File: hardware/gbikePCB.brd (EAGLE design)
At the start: 26.7 x 28.3 mm, 19 parts, among them Q1 16M, U1 nRF51822

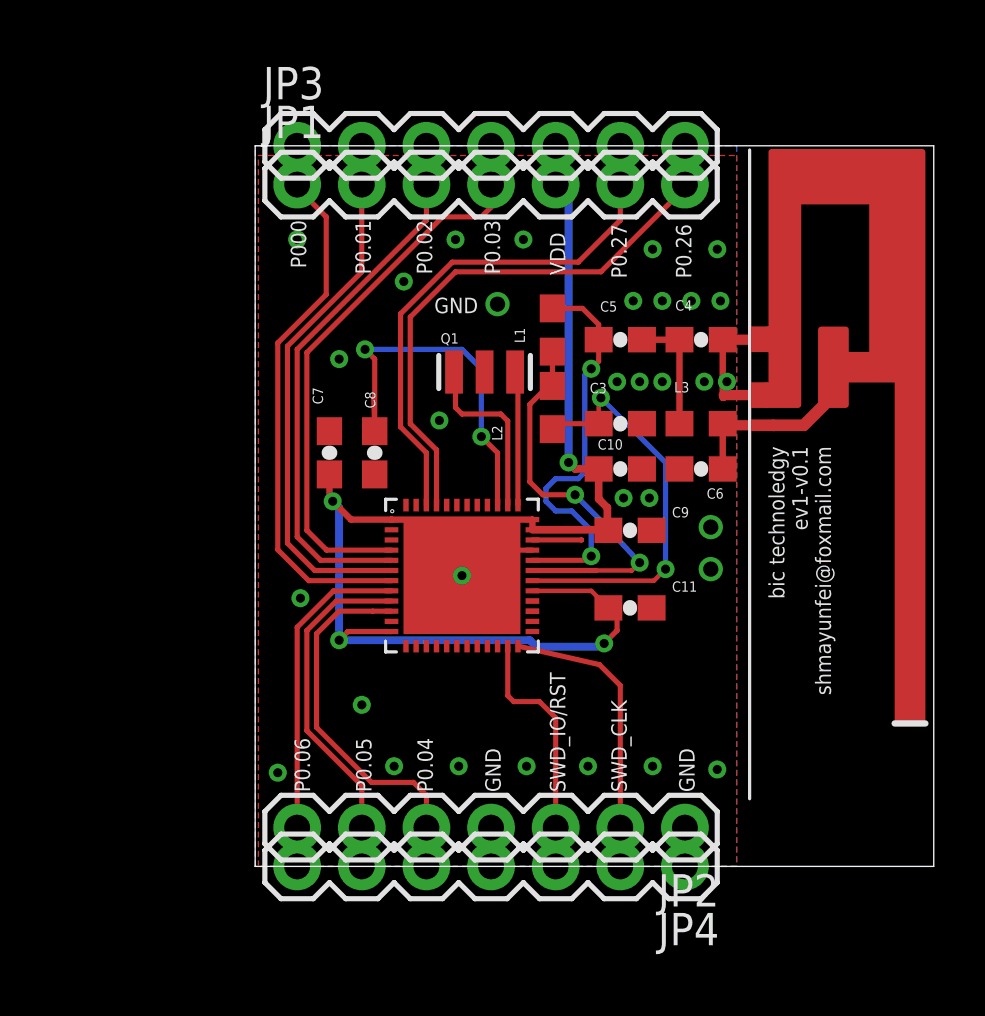
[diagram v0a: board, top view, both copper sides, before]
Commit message: updated pcb file
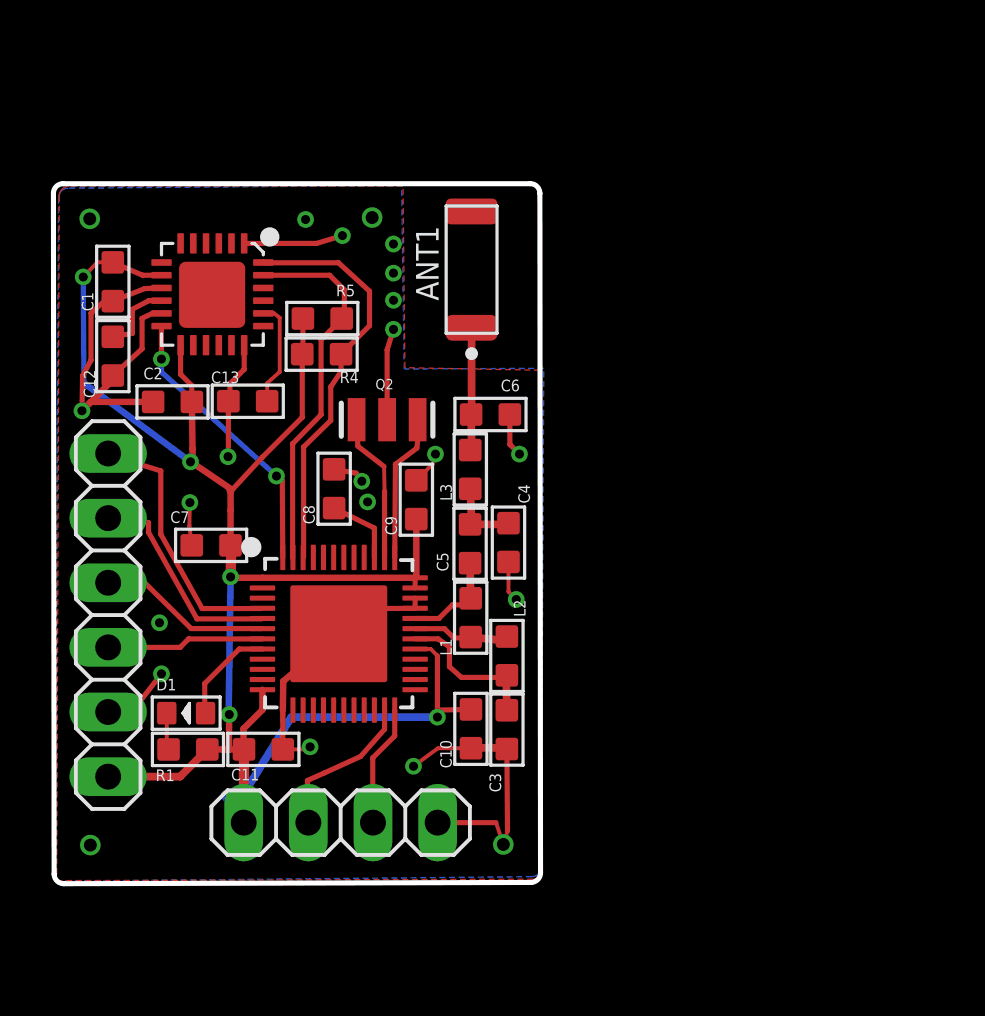
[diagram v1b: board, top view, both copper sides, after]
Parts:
- removed JP3, JP4: (no value), AUSER KJ:1X07
- removed Q1: 16M, APM_v2:DIYDRONES3_RESONATOR-SMD
- removed U$2: ANTENNA_INVERTED_F_ANTENNA-3, nRF51822:ANTENNA_DN007-3
- added ANT1: AN2051, Tiny_BLE_V1.0:CONNECTOR_2P-SMD-L5.05*W.02*H1.07MM
- added C1, C12: 100nF, Tiny_BLE_V1.0:DISCRETE_C0603
- added C13: 2.2nF, Tiny_BLE_V1.0:DISCRETE_C0603
- added C2: 0.1uF, Tiny_BLE_V1.0:DISCRETE_C0603
- added D1: led1, Tiny_BLE_V1.0:DISCRETE_LED-0603
- added NRF51822: nRF51822, nRF51822ModifiedFortValue:NRF51822_NRF51822_QFN48
- added Q2: 16M, APM_v2:DIYDRONES3_RESONATOR-SMD
- added R1: 4.7K, Tiny_BLE_V1.0:DISCRETE_R0603
- added R4, R5: 10k, Tiny_BLE_V1.0:DISCRETE_R0603
- C10, C11, C3, C4, C5, C6, C7, C8, C9: device SparkFun:0603-CAP -> Tiny_BLE_V1.0:DISCRETE_C0603
- JP1: value (none) -> Interface; device AUSER KJ:1X07 -> pinhead:1X06
- JP2: value (none) -> SWD; device AUSER KJ:1X07 -> pinhead:1X04
- L1, L2, L3: device AUSER KJ:0603 -> Tiny_BLE_V1.0:DISCRETE_L0603
- U1: value nRF51822 -> mpu6050; device nRF51822:NRF51822_NORDICSEMI_QFN48 -> nRF51822:TINY_BLE_V1.0_TEMPLATE_QFN24
- moved JP1 18.5 mm to (3.24, 10.6), turned to 270 degrees
- moved C11 15.4 mm to (9.34, 5.36)
- moved U1 14.8 mm to (7.34, 23.2), turned to 270 degrees
- moved JP2 13.5 mm to (12.4, 2.48)
- moved C3 12.8 mm to (18.9, 6.14), turned to 270 degrees
- moved C10 11.8 mm to (17.5, 6.17), turned to 270 degrees
- moved L1 11.8 mm to (17.5, 10.5)
- moved C4 11.0 mm to (19.0, 13.5), turned to 270 degrees
- moved C5 9.96 mm to (17.5, 13.4), turned to 90 degrees
- moved L2 9.92 mm to (18.9, 9.03)
- moved L3 9.25 mm to (17.5, 16.4), turned to 90 degrees
- moved C6 8.55 mm to (18.3, 18.5), turned to 0 degrees
- moved C9 8.48 mm to (15.4, 15.2), turned to 90 degrees
- moved C7 5.91 mm to (7.29, 13.4), turned to 180 degrees
- moved C8 2.13 mm to (12.1, 15.6), turned to 90 degrees
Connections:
- removed net N$1: Q1.3, U1.38
- removed net N$14: JP1.1, JP3.1, U1.7
- removed net N$15: JP2.7, JP4.7, U1.8
- removed net N$16: JP2.6, JP4.6, U1.9
- new net IMU_INT: NRF51822.P48, U1.12
- new net N$18: C12.1, U1.10
- new net N$19: C13.1, U1.20
- new net P04: D1.+, NRF51822.P8
- new net SCL: NRF51822.P47, R5.2, U1.23
- new net SDA: NRF51822.P46, R4.2, U1.24
- net N$10: now also JP1.2, NRF51822.P5; no longer JP1.4, JP3.4, U1.4
- net N$11: now also NRF51822.P6; no longer JP3.3, U1.5
- net N$12: now also NRF51822.P31; no longer U1.31
- net N$13: now also JP1.4, NRF51822.P7; no longer JP1.2, JP3.2, U1.6
- net N$17: now also D1.-, R1.1; no longer JP2.5, JP4.5, U1.10
- net N$2: now also JP1.1, NRF51822.P4; no longer Q1.1, U1.37
- net N$28: now also NRF51822.P23; no longer JP4.3, U1.23
- net N$29: now also NRF51822.P24; no longer JP4.2, U1.24
- net N$3: now also NRF51822.P30; no longer U1.30
- net N$4: now also NRF51822.P38, Q2.3; no longer JP1.7, JP3.7, U1.45
- net N$5: now also NRF51822.P39; no longer U1.39
- net N$6: now also NRF51822.P32; no longer U1.32
- net N$8: now also ANT1.1; no longer U$2.FEED
- net N$9: now also NRF51822.P37, Q2.1; no longer JP1.6, JP3.6, U1.46
- net VDD: now also C1.1, C2.2, JP1.6, JP2.4, NRF51822.P1, NRF51822.P12, NRF51822.P29, NRF51822.P35, NRF51822.P36, R1.2, R4.1, R5.1, U1.13, U1.8; no longer JP1.5, JP3.5, U1.1, U1.12, U1.29, U1.35, U1.36
- net VSS: now also C1.2, C12.2, C13.2, C2.1, JP1.5, NRF51822.P13, NRF51822.P33, NRF51822.P34, NRF51822.VSS, Q2.2, U1.1, U1.11, U1.18, U1.9; no longer JP2.4, JP4.1, JP4.4, Q1.2, U$2.GND, U$2.GND@1, U1.13, U1.33, U1.34, U1.GND
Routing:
- net VSS: track 11.0 -> 59.8 mm, vias 32 -> 22
- net N$14: track 22.1 -> 0.00 mm
- net VDD: track 55.0 -> 76.7 mm, vias 4 -> 5
- net N$4: track 22.4 -> 5.92 mm
- net SDA: track 0.00 -> 16.3 mm
- net N$13: track 21.4 -> 6.20 mm
- net N$9: track 21.0 -> 6.08 mm
- net SCL: track 0.00 -> 14.9 mm
- net N$11: track 21.6 -> 6.80 mm
- net N$10: track 22.7 -> 8.53 mm
- net N$16: track 14.0 -> 0.00 mm
- net N$17: track 15.2 -> 1.45 mm
- net N$15: track 13.7 -> 0.00 mm
- net N$5: track 15.2 -> 2.92 mm, vias 2 -> 0
- net N$6: track 16.0 -> 3.95 mm, vias 2 -> 0
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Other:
- board size 26.7 x 28.3 mm -> 19.1 x 27.5 mm
- board text added: "Blue Magic v0.2 shmayunfei@qq.com Shanghai Geek Tribe"
- board text added: "P0"
- board text added: "P1"
- board text added: "P2"
- board text added: "P3"
- board text added: "SWCLK"
- board text added: "SWDIO"
- board text added: "VCC"
- board text added: "vcc"
- board text removed: "P0.01"
- board text removed: "P0.02"
- board text removed: "P0.03"
- board text removed: "P0.04"
- board text removed: "P0.05"
- board text removed: "P0.06"
- board text removed: "P0.26"
- board text removed: "P0.27"
- board text removed: "P000"
- board text removed: "SWD_CLK"
- board text removed: "SWD_IO/RST"
- board text removed: "VDD"
- board text removed: "bic technoledgy ev1-v0.1 shmayunfei@foxmail.com"
